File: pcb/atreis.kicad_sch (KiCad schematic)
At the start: 114 parts, among them SW1 SW_Push, U1 Elite-C

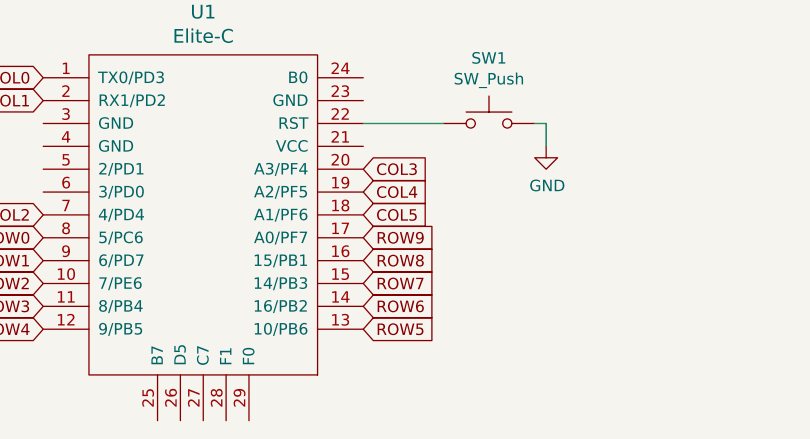
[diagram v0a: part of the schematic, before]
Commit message: Completed tracks and edge. Cleaned up drawings.
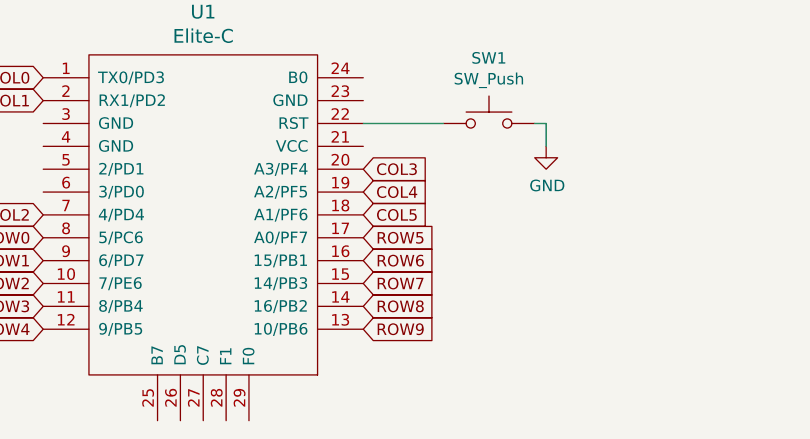
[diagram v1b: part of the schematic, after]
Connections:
- net ROW5: now also U1.17 (A0/PF7); no longer U1.13 (10/PB6)
- net ROW6: now also U1.16 (15/PB1); no longer U1.14 (16/PB2)
- net ROW8: now also U1.14 (16/PB2); no longer U1.16 (15/PB1)
- net ROW9: now also U1.13 (10/PB6); no longer U1.17 (A0/PF7)
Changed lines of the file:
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@@
     )
   )
-  (global_label "ROW5" (shape input) (at 111.76 170.18 0) (fields_autoplaced)
+  (global_label "ROW5" (shape input) (at 111.76 160.02 0) (fields_autoplaced)
     (effects (font (size 1.27 1.27)) (justify left))
-    (property "Intersheet References" "${INTERSHEET_REFS}" (id 0) (at -57.15 3.81 0)
+    (property "Intersheet References" "${INTERSHEET_REFS}" (id 0) (at -57.15 -6.35 0)
       (effects (font (size 1.27 1.27)) hide)
     )
@@
     )
   )
-  (global_label "ROW8" (shape input) (at 111.76 162.56 0) (fields_autoplaced)
+  (global_label "ROW8" (shape input) (at 111.76 167.64 0) (fields_autoplaced)
     (effects (font (size 1.27 1.27)) (justify left))
-    (property "Intersheet References" "${INTERSHEET_REFS}" (id 0) (at -57.15 -11.43 0)
+    (property "Intersheet References" "${INTERSHEET_REFS}" (id 0) (at -57.15 -6.35 0)
       (effects (font (size 1.27 1.27)) hide)
     )
@@
     )
   )
-  (global_label "ROW9" (shape input) (at 111.76 160.02 0) (fields_autoplaced)
+  (global_label "ROW9" (shape input) (at 111.76 170.18 0) (fields_autoplaced)
     (effects (font (size 1.27 1.27)) (justify left))
-    (property "Intersheet References" "${INTERSHEET_REFS}" (id 0) (at -57.15 -16.51 0)
+    (property "Intersheet References" "${INTERSHEET_REFS}" (id 0) (at -57.15 -6.35 0)
       (effects (font (size 1.27 1.27)) hide)
     )
@@
     )
   )
-  (global_label "ROW6" (shape input) (at 111.76 167.64 0) (fields_autoplaced)
+  (global_label "ROW6" (shape input) (at 111.76 162.56 0) (fields_autoplaced)
     (effects (font (size 1.27 1.27)) (justify left))
-    (property "Intersheet References" "${INTERSHEET_REFS}" (id 0) (at -57.15 -1.27 0)
+    (property "Intersheet References" "${INTERSHEET_REFS}" (id 0) (at -57.15 -6.35 0)
       (effects (font (size 1.27 1.27)) hide)
     )
